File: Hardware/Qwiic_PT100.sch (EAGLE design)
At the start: 45 parts, among them IC1 ADS122C04IPWR, J2 QWIIC_RIGHT_ANGLE, J3 PTH, J4 QWIIC_RIGHT_ANGLE

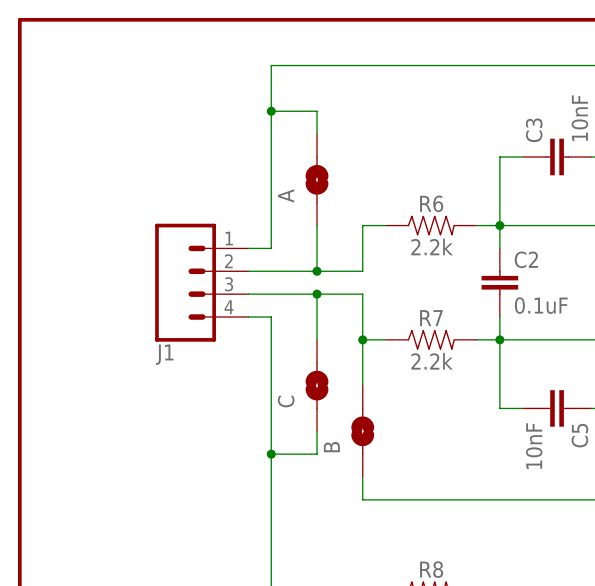
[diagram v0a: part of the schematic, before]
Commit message: Tweaks
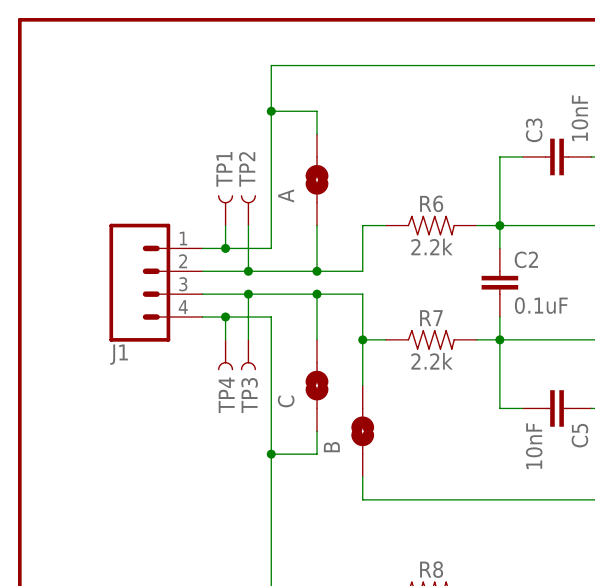
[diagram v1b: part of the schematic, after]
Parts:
- added TP1, TP2, TP3, TP4: TEST-POINTTP_15TH_THRU, SparkFun-Connectors:TEST-POINTTP_15TH_THRU
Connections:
- net AIN3: now also TP1.1
- net N$1: now also TP2.1
- net N$5: now also TP3.1
- net N$6: now also TP4.1
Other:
- moved on the sheet: J1
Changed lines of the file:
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@@
 <part name="GND13" library="SparkFun-PowerSymbols" deviceset="GND" device=""/>
 <part name="SUPPLY5" library="SparkFun-PowerSymbols" deviceset="3.3V" device=""/>
+<part name="TP1" library="SparkFun-Connectors" deviceset="TEST-POINT" device="TP_15TH_THRU"/>
+<part name="TP2" library="SparkFun-Connectors" deviceset="TEST-POINT" device="TP_15TH_THRU"/>
+<part name="TP3" library="SparkFun-Connectors" deviceset="TEST-POINT" device="TP_15TH_THRU"/>
+<part name="TP4" library="SparkFun-Connectors" deviceset="TEST-POINT" device="TP_15TH_THRU"/>
 </parts>
 <sheets>
@@
 <attribute name="VALUE" x="165.1" y="106.934" size="1.778" layer="96" align="bottom-center"/>
 </instance>
-<instance part="J1" gate="J1" x="20.32" y="157.48" smashed="yes" rot="MR180">
-<attribute name="VALUE" x="15.24" y="164.846" size="1.778" layer="96" font="vector" rot="MR180"/>
-<attribute name="NAME" x="15.24" y="149.352" size="1.778" layer="95" font="vector" rot="MR180"/>
+<instance part="J1" gate="J1" x="15.24" y="157.48" smashed="yes" rot="MR180">
+<attribute name="VALUE" x="10.16" y="164.846" size="1.778" layer="96" font="vector" rot="MR180"/>
+<attribute name="NAME" x="10.16" y="149.352" size="1.778" layer="95" font="vector" rot="MR180"/>
 </instance>
 <instance part="GND11" gate="1" x="172.72" y="68.58" smashed="yes">
@@
 <instance part="SUPPLY5" gate="G$1" x="182.88" y="124.46" smashed="yes">
 <attribute name="VALUE" x="182.88" y="127.254" size="1.778" layer="96" align="bottom-center"/>
+</instance>
+<instance part="TP1" gate="G$1" x="22.86" y="162.56" smashed="yes" rot="R90">
+<attribute name="NAME" x="23.622" y="166.878" size="1.778" layer="95" font="vector" rot="R90"/>
+</instance>
+<instance part="TP2" gate="G$1" x="25.4" y="162.56" smashed="yes" rot="R90">
+<attribute name="NAME" x="26.162" y="166.878" size="1.778" layer="95" font="vector" rot="R90"/>
+</instance>
+<instance part="TP3" gate="G$1" x="25.4" y="149.86" smashed="yes" rot="R270">
+<attribute name="NAME" x="24.638" y="145.796" size="1.778" layer="95" font="vector" rot="R270"/>
+</instance>
+<instance part="TP4" gate="G$1" x="22.86" y="149.86" smashed="yes" rot="R270">
+<attribute name="NAME" x="22.098" y="145.796" size="1.778" layer="95" font="vector" rot="R270"/>
 </instance>
 </instances>
@@
 <segment>
 <pinref part="J1" gate="J1" pin="1"/>
-<wire x1="25.4" y1="160.02" x2="27.94" y2="160.02" width="0.1524" layer="91"/>
+<wire x1="20.32" y1="160.02" x2="22.86" y2="160.02" width="0.1524" layer="91"/>
+<wire x1="22.86" y1="160.02" x2="27.94" y2="160.02" width="0.1524" layer="91"/>
 <wire x1="27.94" y1="160.02" x2="27.94" y2="175.26" width="0.1524" layer="91"/>
 <label x="104.14" y="180.34" size="1.27" layer="95" xref="yes"/>
@@
 <wire x1="33.02" y1="175.26" x2="27.94" y2="175.26" width="0.1524" layer="91"/>
 <junction x="27.94" y="175.26"/>
+<pinref part="TP1" gate="G$1" pin="1"/>
+<wire x1="22.86" y1="162.56" x2="22.86" y2="160.02" width="0.1524" layer="91"/>
+<junction x="22.86" y="160.02"/>
 </segment>
 </net>
@@
 <segment>
 <pinref part="J1" gate="J1" pin="2"/>
+<wire x1="20.32" y1="157.48" x2="25.4" y2="157.48" width="0.1524" layer="91"/>
 <wire x1="25.4" y1="157.48" x2="33.02" y2="157.48" width="0.1524" layer="91"/>
 <wire x1="33.02" y1="157.48" x2="38.1" y2="157.48" width="0.1524" layer="91"/>
@@
 <wire x1="33.02" y1="162.56" x2="33.02" y2="157.48" width="0.1524" layer="91"/>
 <junction x="33.02" y="157.48"/>
+<pinref part="TP2" gate="G$1" pin="1"/>
+<wire x1="25.4" y1="162.56" x2="25.4" y2="157.48" width="0.1524" layer="91"/>
+<junction x="25.4" y="157.48"/>
 </segment>
 </net>
@@
 <segment>
 <pinref part="J1" gate="J1" pin="3"/>
+<wire x1="20.32" y1="154.94" x2="25.4" y2="154.94" width="0.1524" layer="91"/>
 <wire x1="25.4" y1="154.94" x2="33.02" y2="154.94" width="0.1524" layer="91"/>
 <wire x1="33.02" y1="154.94" x2="38.1" y2="154.94" width="0.1524" layer="91"/>
@@
 <wire x1="38.1" y1="144.78" x2="38.1" y2="149.86" width="0.1524" layer="91"/>
 <junction x="38.1" y="149.86"/>
+<pinref part="TP3" gate="G$1" pin="1"/>
+<wire x1="25.4" y1="149.86" x2="25.4" y2="154.94" width="0.1524" layer="91"/>
+<junction x="25.4" y="154.94"/>
 </segment>
 </net>
@@
 <segment>
 <pinref part="J1" gate="J1" pin="4"/>
-<wire x1="25.4" y1="152.4" x2="27.94" y2="152.4" width="0.1524" layer="91"/>
+<wire x1="20.32" y1="152.4" x2="22.86" y2="152.4" width="0.1524" layer="91"/>
 <pinref part="R9" gate="G$1" pin="2"/>
+<wire x1="22.86" y1="152.4" x2="27.94" y2="152.4" width="0.1524" layer="91"/>
 <wire x1="27.94" y1="152.4" x2="27.94" y2="137.16" width="0.1524" layer="91"/>
 <pinref part="R8" gate="G$1" pin="1"/>
@@
 <wire x1="33.02" y1="137.16" x2="27.94" y2="137.16" width="0.1524" layer="91"/>
 <junction x="27.94" y="137.16"/>
-</segment>
-</net>
+<pinref part="TP4" gate="G$1" pin="1"/>
+<wire x1="22.86" y1="149.86" x2="22.86" y2="152.4" width="0.1524" layer="91"/>
+<junction x="22.86" y="152.4"/>
+</segment>
+</net>
